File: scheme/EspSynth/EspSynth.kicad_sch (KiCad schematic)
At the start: 18 parts, among them SW1 SW_Push, SW10 SW_Push, SW11 SW_Push, SW12 SW_Push, SW2 SW_Push, SW3 SW_Push, SW4 SW_Push, SW5 SW_Push, SW6 SW_Push, SW7 SW_Push, SW8 SW_Push, SW9 SW_Push

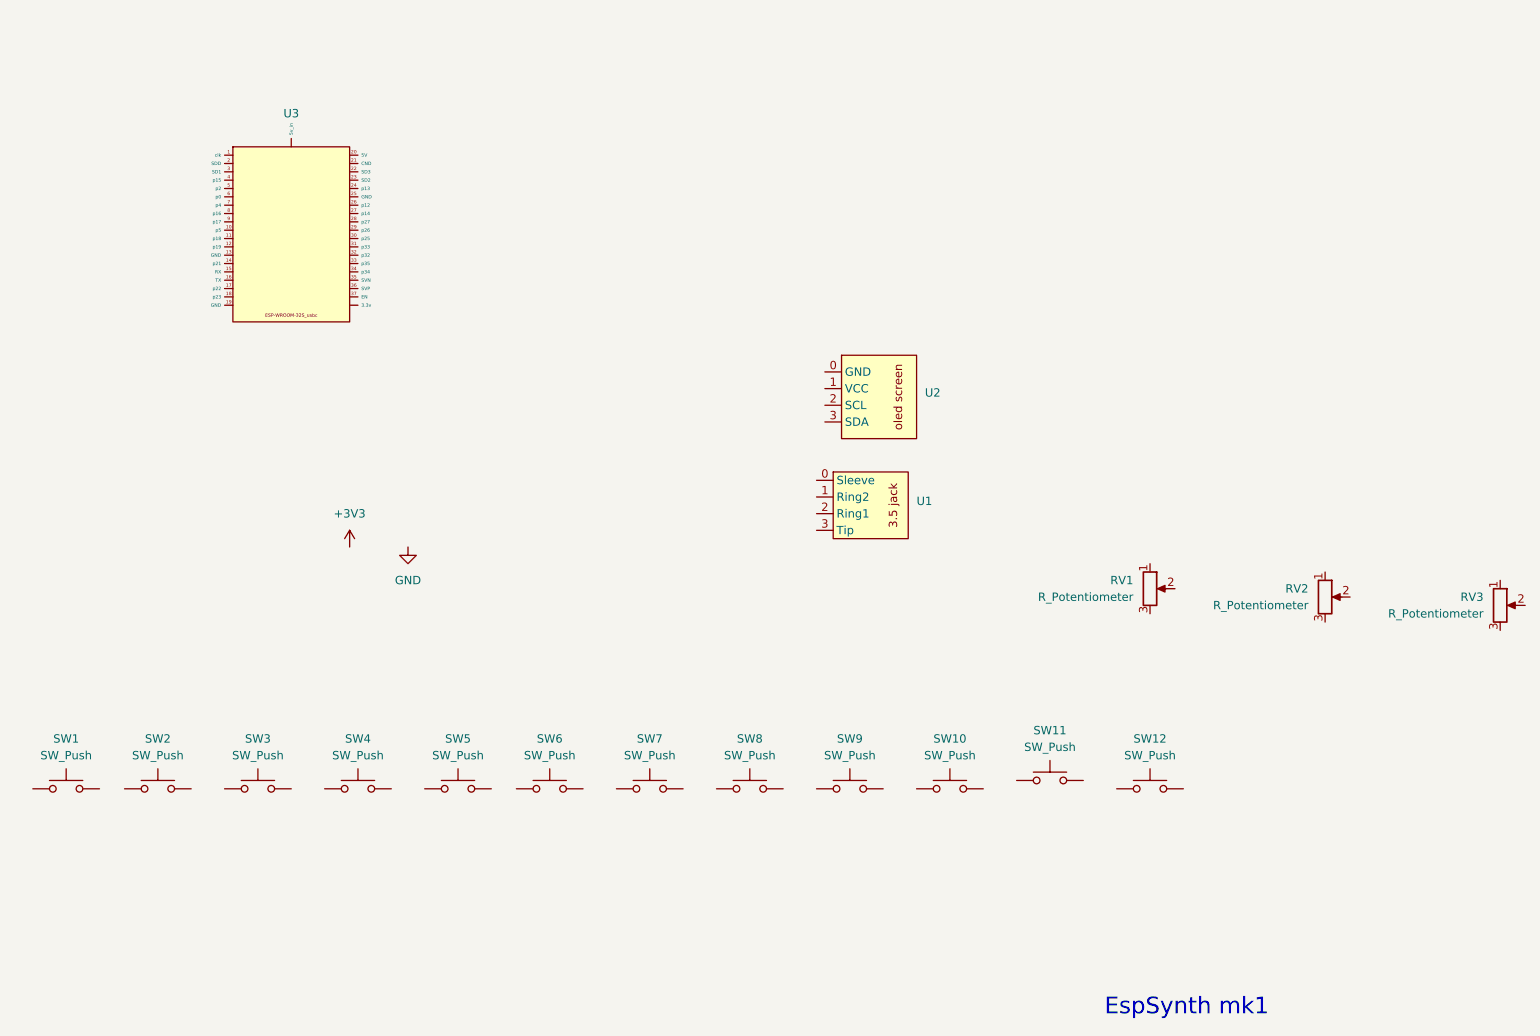
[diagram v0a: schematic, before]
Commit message: connections done
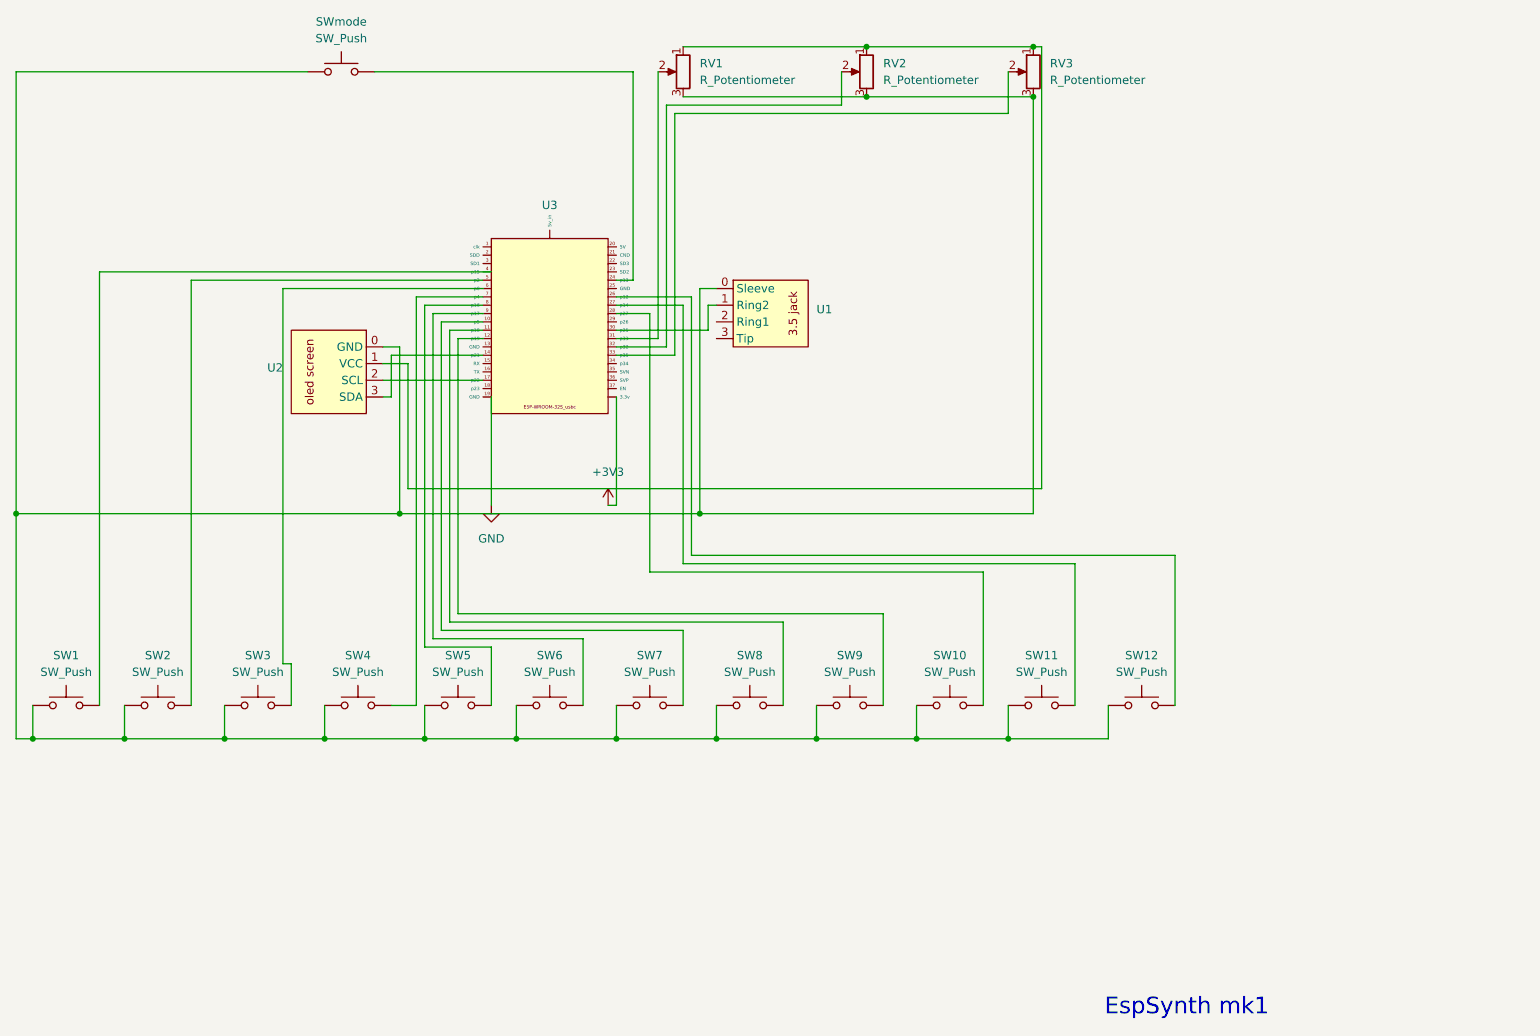
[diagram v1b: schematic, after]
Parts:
- added SWmode: SW_Push, symbol Switch:SW_Push
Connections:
- net GND: now also U3.19 (GND)
- net at SW6.1: now also RV1.3, RV2.3, RV3.3, SW1.1, SW10.1, SW11.1, SW12.1, SW2.1, SW3.1, SW4.1, SW5.1, SW7.1, SW8.1, SW9.1, U1.0 (Sleeve), U2.0 (GND), SWmode.1
- net at RV1.1: now also RV2.1, RV3.1, U2.1 (VCC)
- net at U3.4 (p15): now also SW1.2
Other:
- moved on the sheet: RV1, RV2, RV3, SW1, SW10, SW11, SW12, SW2, SW3, SW4, SW5, SW6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
